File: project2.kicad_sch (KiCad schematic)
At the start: 28 parts, among them J1 USB_C_Receptacle_PowerOnly_6P, J2 Conn_01x01_Socket, J3 Conn_01x01_Socket, J4 Conn_01x01_Socket, J5 Conn_01x01_Socket, Q1 FS8205A, Q2 DW01A, SW1 SW_Nidec_CAS-120A1, U1 TP4056-42-ESOP8, U2 MT3608

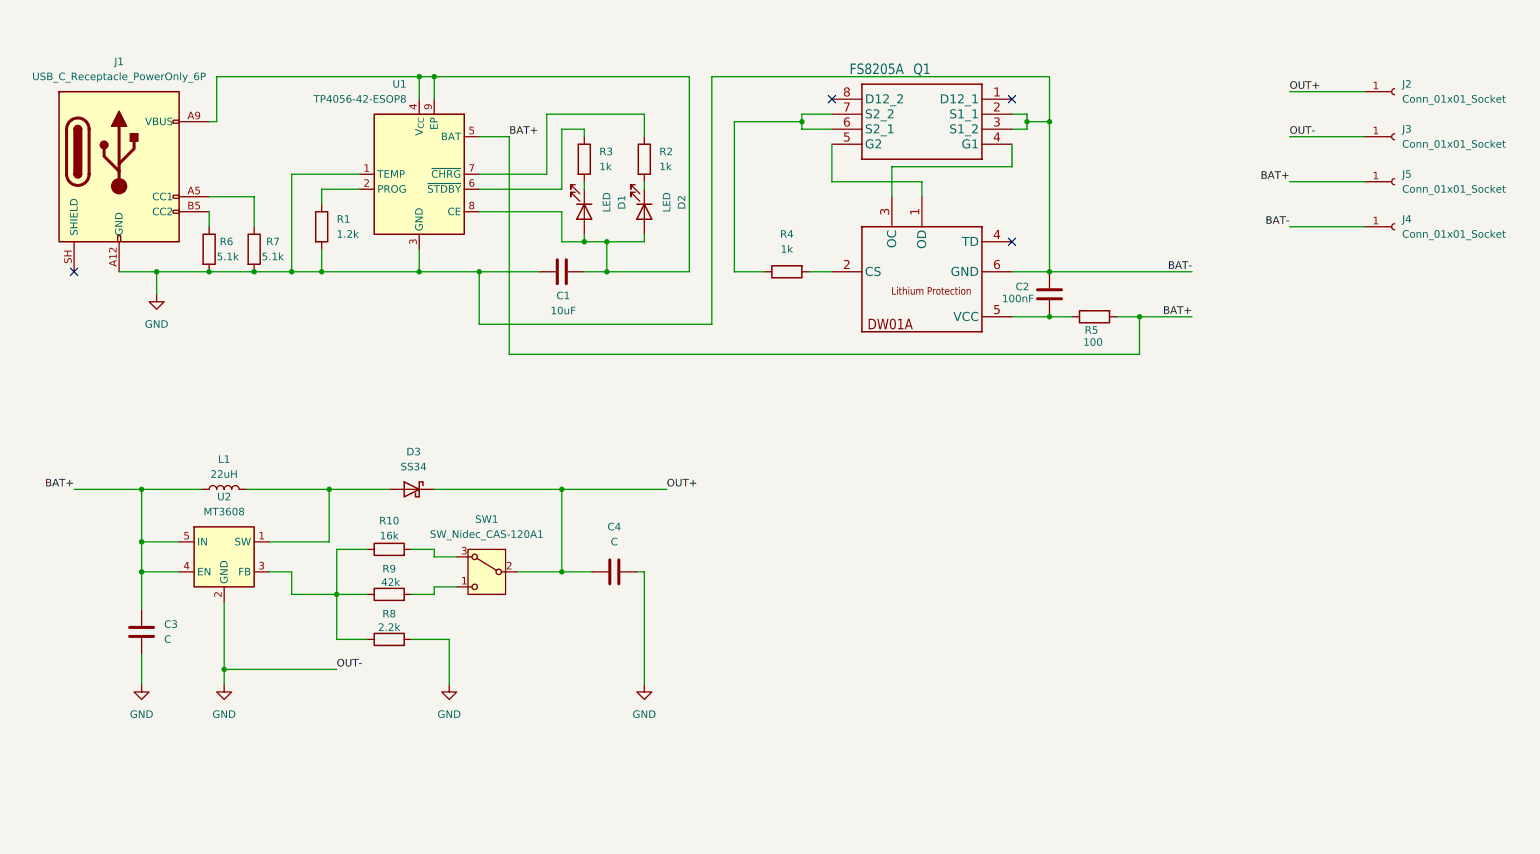
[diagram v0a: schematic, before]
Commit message: PCB created
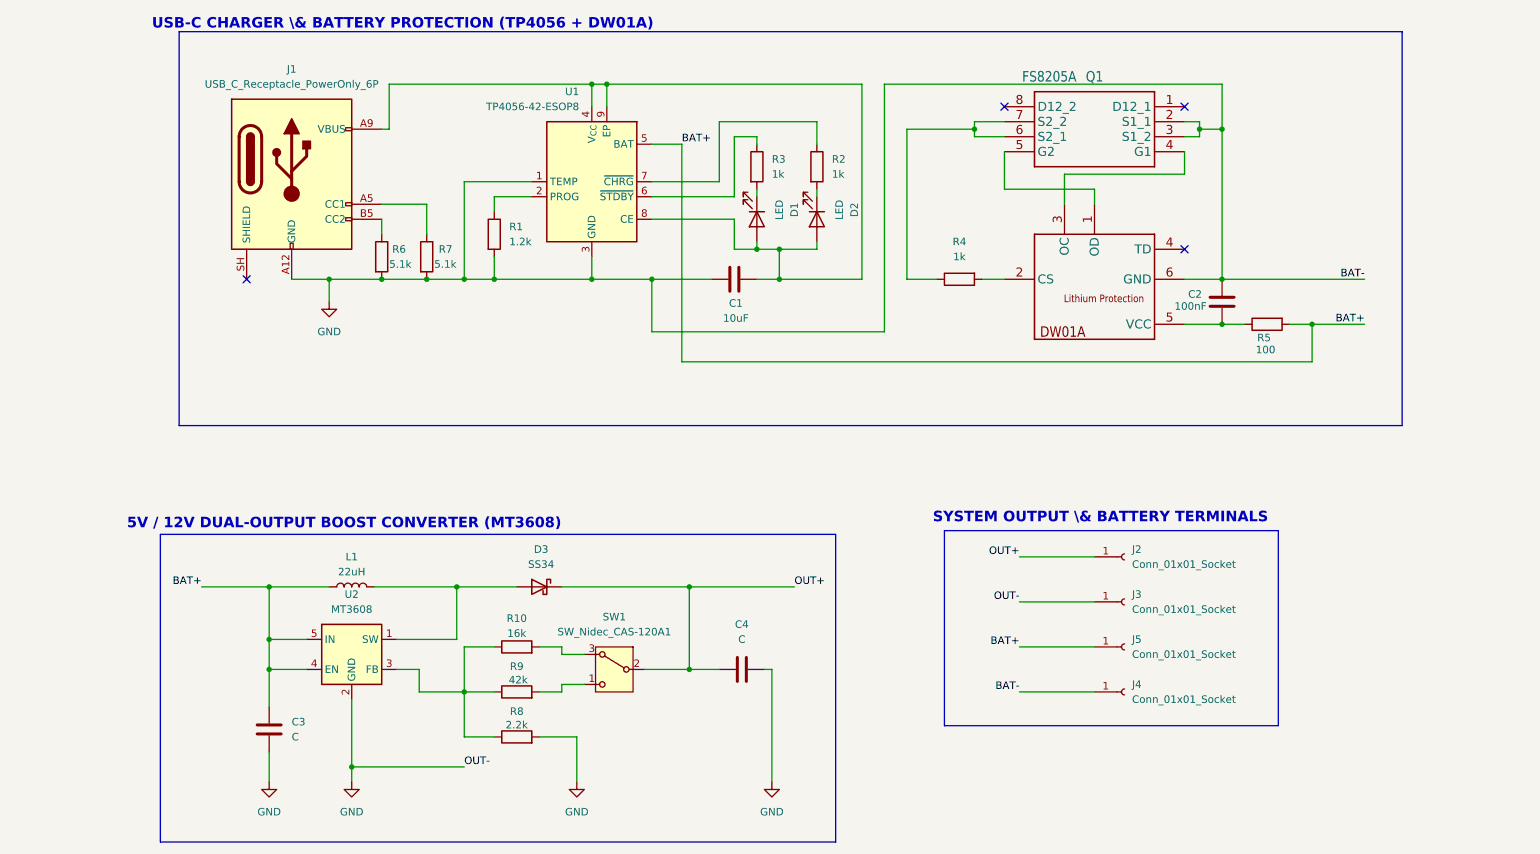
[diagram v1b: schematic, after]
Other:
- note added: "5V / 12V DUAL-OUTPUT BOOST CONVERTER (MT3608)"
- note added: "SYSTEM OUTPUT \& BATTERY TERMINALS"
- note added: "USB-C CHARGER \& BATTERY PROTECTION (TP4056 + DW01A)"
- company: (none) -> Devendra Kashyap
- title: (none) -> Li-Po Battery Charger & Selectable 5V/12V Boost Module
- moved on the sheet: C1, C2, C3, C4, D1, D2, D3, J1, J2, J3, J4, J5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
